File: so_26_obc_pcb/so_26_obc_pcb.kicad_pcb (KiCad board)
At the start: 4 copper layers, 90.2 x 95.9 mm, 52 parts, among them J1 Conn_02x06_Odd_Even, J10 Conn_01x04, J2 Conn_02x12_Odd_Even, J3 Conn_01x04, J4 Conn_01x03, J5 Conn_01x02, J6 Conn_01x02, J7 Conn_01x02, J8 Conn_01x03, SW1 SW_Push, U1 STM32G431RBTx, U2 TPT3232A-TS3R, U3 PCT2075, U4 MPRLS0025, U5 LSM6DS3, U6 MEM2067-02-180-00-A

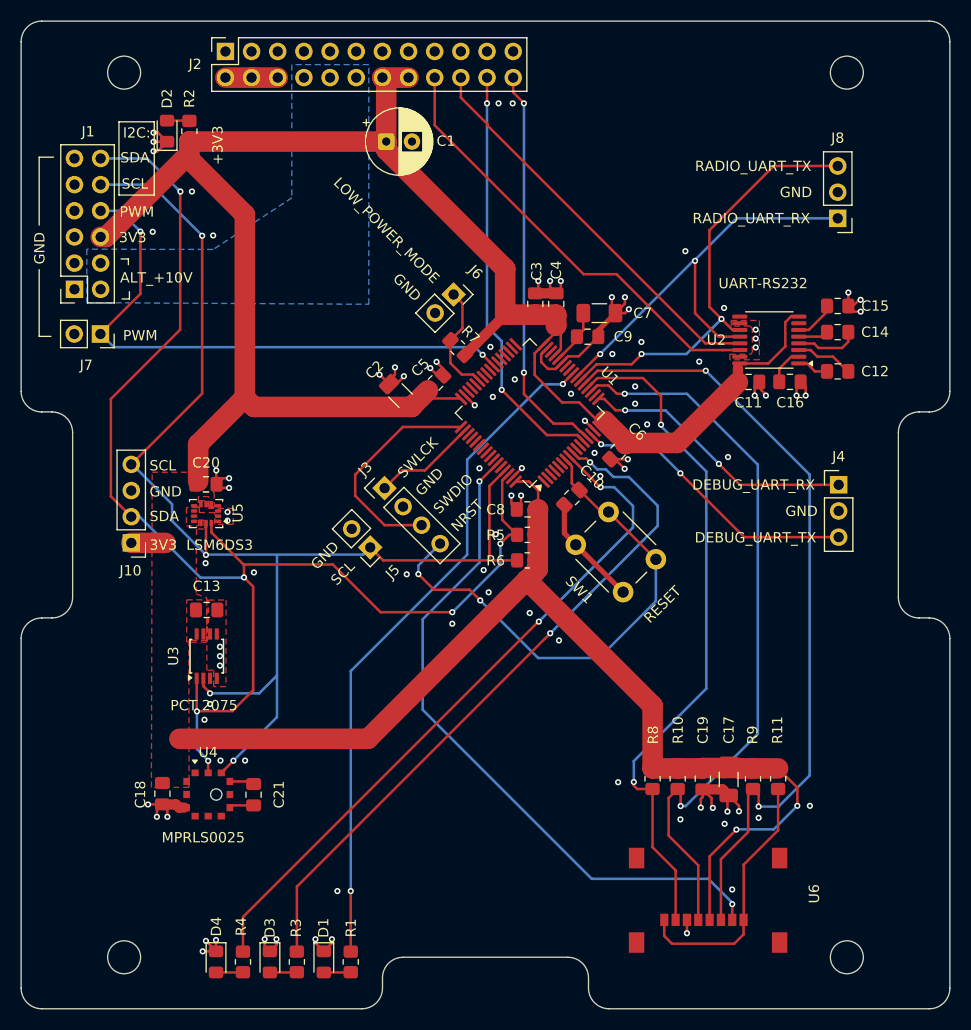
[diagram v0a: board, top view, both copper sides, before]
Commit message: PCB: Finished rev2, I think
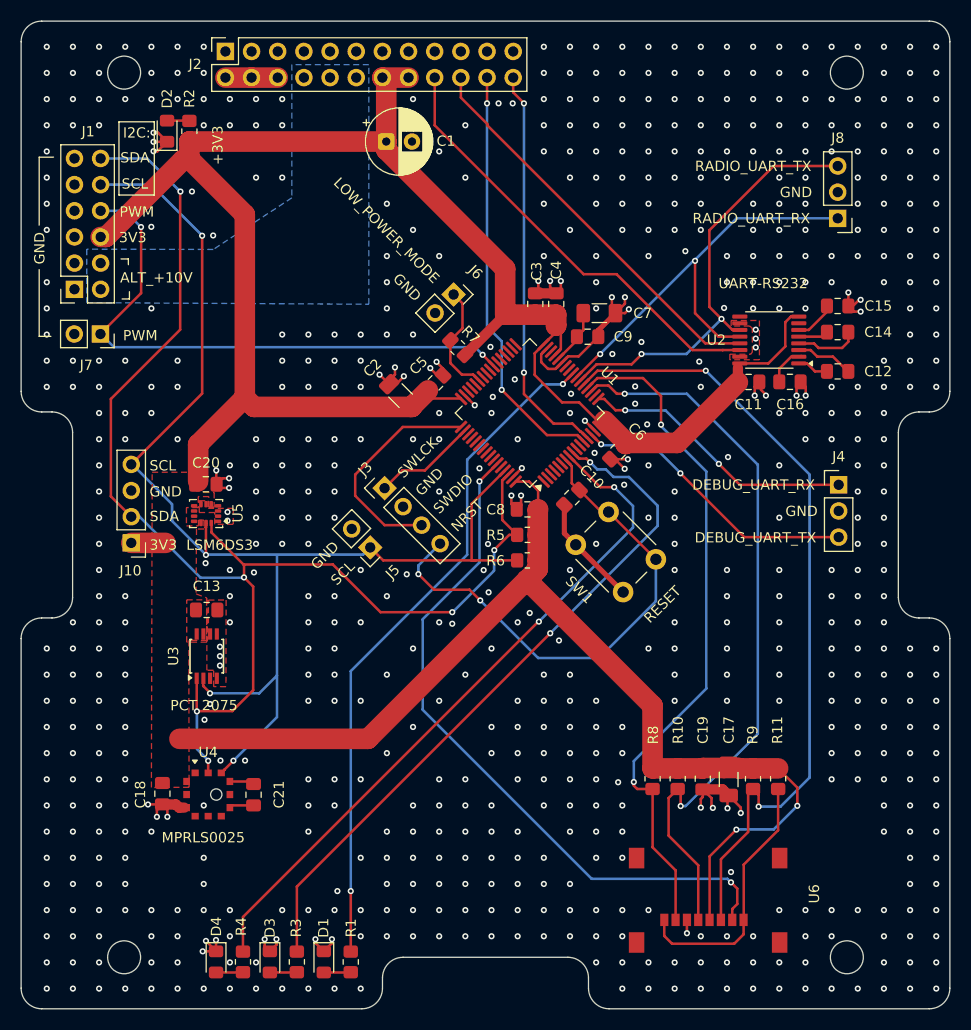
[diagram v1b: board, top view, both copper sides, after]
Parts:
- added G***: LOGO, LOGO, B.Cu at (131.5, 125.4)
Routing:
- net /SD_CS: track 66.4 -> 67.9 mm
- net /BOOT0: track 124.7 -> 125.7 mm
- net GND: vias 95 -> 692
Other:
- board text added: "I wanna be a teddy bear ...being a human is unBEARable!"
- board text added: "Regine Angermo Birkely Suborbital_CyanoSat_25/26 01.03.2026 SO26 - OBC Rev 2"
- board text removed: "SO26 - OBC Rev 1 Regine Angermo Birkely 11.02.26"
